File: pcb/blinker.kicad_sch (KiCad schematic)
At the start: 9 parts, among them J1 ISP, U1 ATtiny10-TS

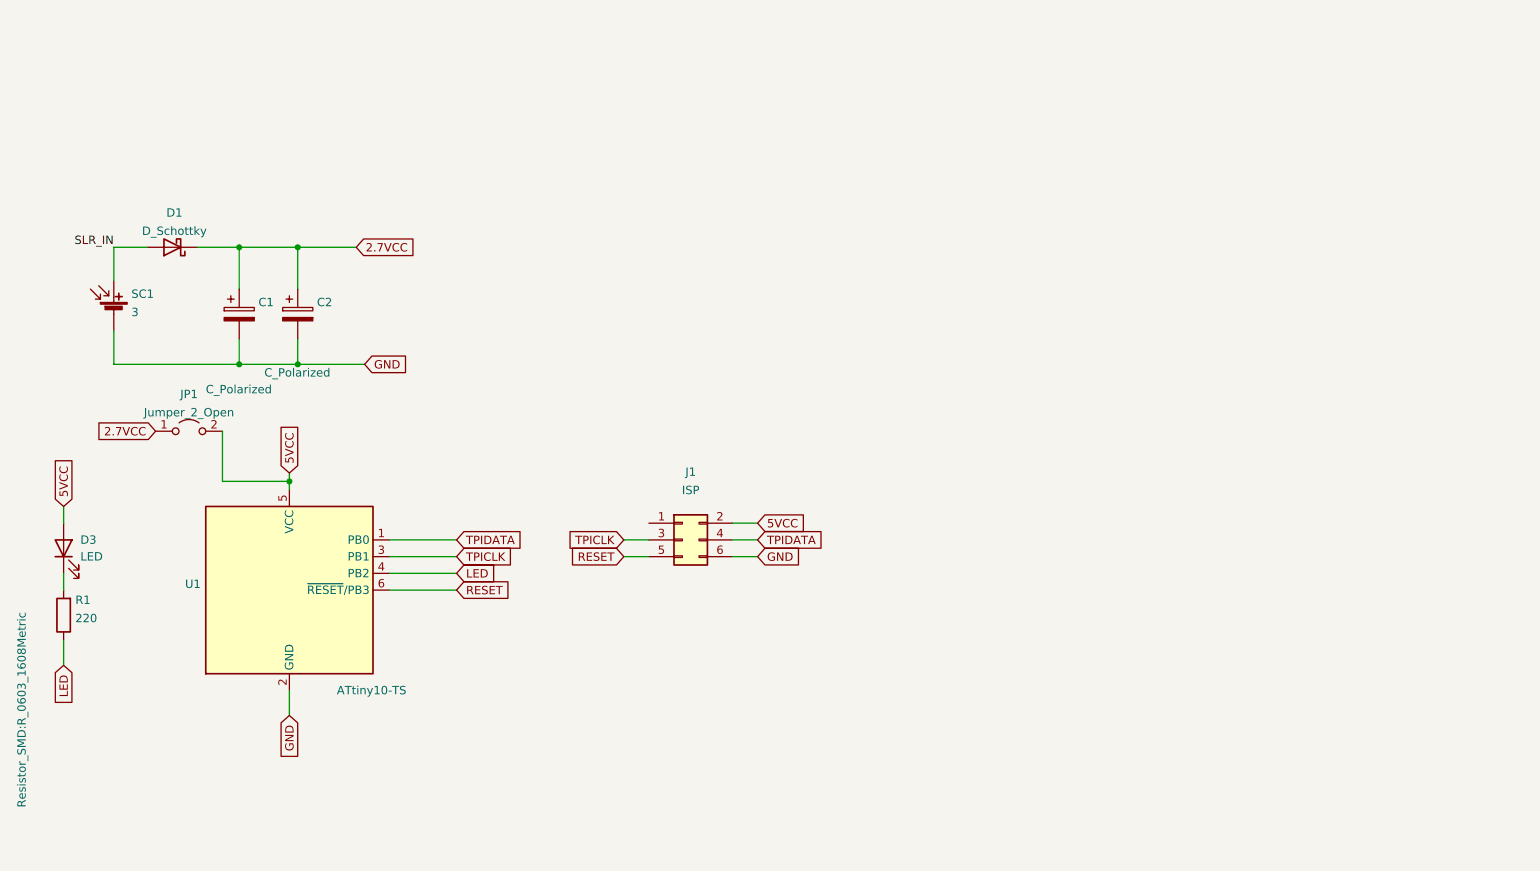
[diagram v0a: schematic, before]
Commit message: Making progress
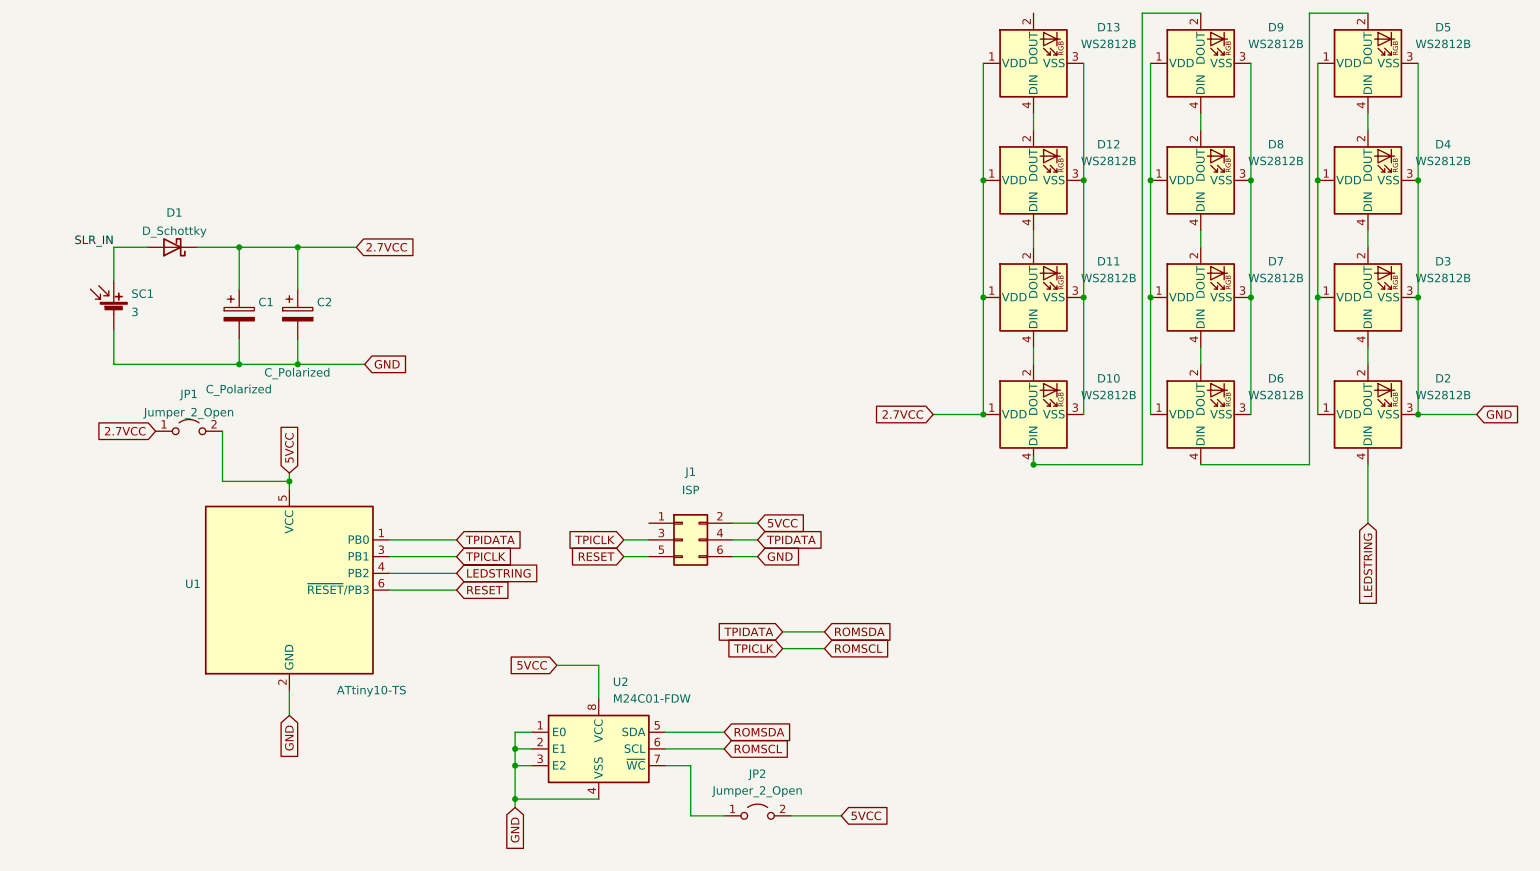
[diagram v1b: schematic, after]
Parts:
- removed D3: LED, LED_SMD:LED_0603_1608Metric, symbol Device:LED
- removed R1: 220, Resistor_SMD:R_0603_1608Metric, symbol Device:R
- added D10, D11, D12, D13, D2, D3, D4, D5, D6, D7, D8, D9: WS2812B, LED_SMD:LED_Wurth_150044M155260, symbol LED:WS2812B
- added JP2: Jumper_2_Open, Jumper:SolderJumper-2_P1.3mm_Open_TrianglePad1.0x1.5mm, symbol Jumper:Jumper_2_Open
- added U2: M24C01-FDW, Package_SO:TSSOP-8_4.4x3mm_P0.65mm, symbol Memory_EEPROM:M24C01-FDW
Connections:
- net 2.7VCC: now also D10.1 (VDD), D11.1 (VDD), D12.1 (VDD), D13.1 (VDD)
- net 5VCC: now also JP2.2 (B), U2.8 (VCC)
- net GND: now also D2.3 (VSS), D3.3 (VSS), D4.3 (VSS), D5.3 (VSS), U2.1 (E0), U2.2 (E1), U2.3 (E2), U2.4 (VSS)
- net LED renamed LEDSTRING
- net LEDSTRING: now also D2.4 (DIN)
- net TPICLK renamed ROMSCL
- net ROMSCL: now also U2.6 (SCL)
- net TPIDATA renamed ROMSDA
- net ROMSDA: now also U2.5 (SDA)
- new net: D6.1 (VDD), D7.1 (VDD), D8.1 (VDD), D9.1 (VDD)
- new net: D10.4 (DIN), D9.2 (DOUT)
- new net: D6.3 (VSS), D7.3 (VSS), D8.3 (VSS), D9.3 (VSS)
- new net: D8.2 (DOUT), D9.4 (DIN)
- new net: D12.2 (DOUT), D13.4 (DIN)
- new net: D10.3 (VSS), D11.3 (VSS), D12.3 (VSS), D13.3 (VSS)
- new net: D11.2 (DOUT), D12.4 (DIN)
- new net: JP2.1 (A), U2.7 (~{WC})
- new net: D2.1 (VDD), D3.1 (VDD), D4.1 (VDD), D5.1 (VDD)
- new net: D5.2 (DOUT), D6.4 (DIN)
- new net: D4.2 (DOUT), D5.4 (DIN)
- new net: D2.2 (DOUT), D3.4 (DIN)
- new net: D10.2 (DOUT), D11.4 (DIN)
- new net: D7.2 (DOUT), D8.4 (DIN)
- new net: D6.2 (DOUT), D7.4 (DIN)
- new net: D3.2 (DOUT), D4.4 (DIN)
